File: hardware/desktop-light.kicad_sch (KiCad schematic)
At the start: 95 parts, among them J1 Conn_01x06, J2 Conn_01x06, J3 USB_B_Micro, J4 Barrel_Jack, J5 Conn_01x06, Q1 BSS138, Q2 BSS138, U1 ESP32-WROOM-32, U2 AMS1117-3.3, U3 CH340C, U4 PCF8523T, Y1 ABS2532768KHZ6T

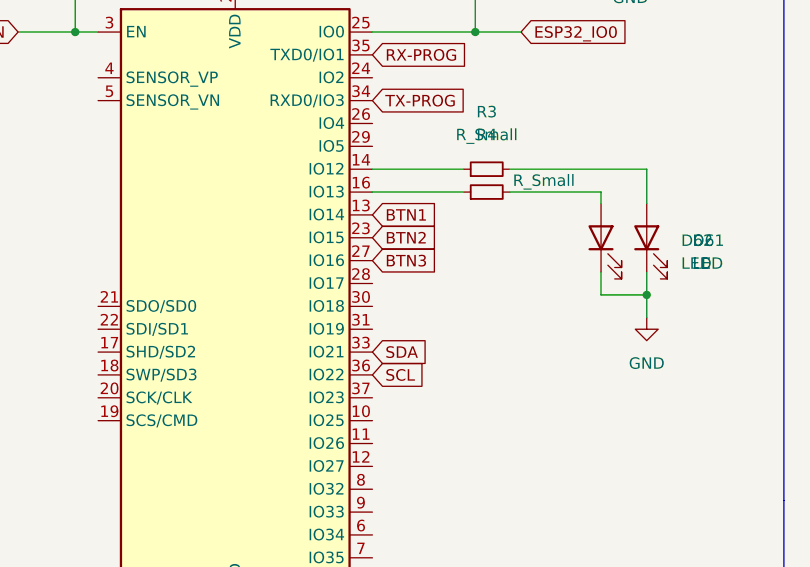
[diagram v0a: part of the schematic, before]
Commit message: add real photos
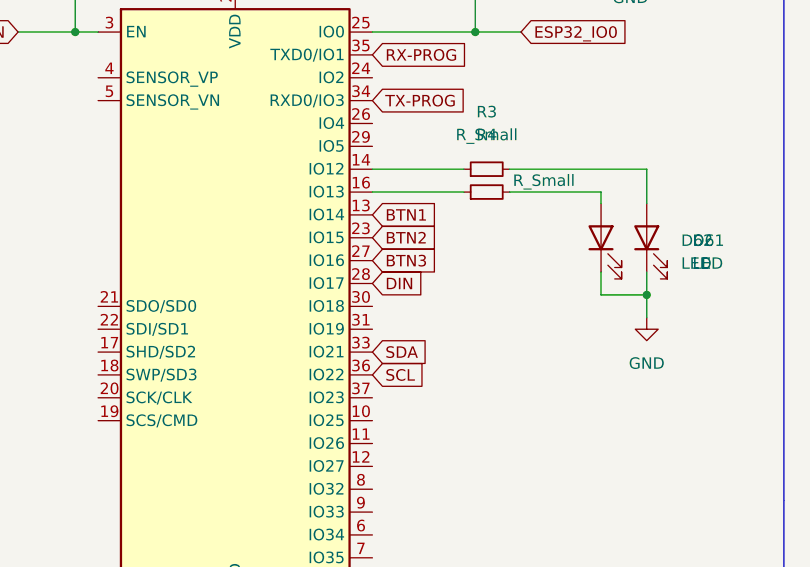
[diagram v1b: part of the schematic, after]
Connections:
- net DIN: now also U1.28 (IO17)
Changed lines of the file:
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@@
+		)
+	)
+	(global_label "DIN"
+		(shape input)
+		(at 351.79 100.33 0)
+		(fields_autoplaced yes)
+		(effects
+			(font
+				(size 1.27 1.27)
+			)
+			(justify left)
+		)
+		(property "Intersheetrefs" "${INTERSHEET_REFS}"
+			(at 357.9805 100.33 0)
+			(effects
+				(font
+					(size 1.27 1.27)
+				)
+				(justify left)
+				(hide yes)
+			)
 		)
 	)
